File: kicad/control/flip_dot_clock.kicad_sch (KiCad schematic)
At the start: 34 parts, among them J1 Conn_01x02_Male, U1 NUCLEO-F303K8-HEADER, U10 Small_7_Seg_FlipDot_Module, U2 SLC03B-05, U3 NCV7719, U4 Small_7_Seg_FlipDot_Module, U5 NCV7719, U6 Small_7_Seg_FlipDot_Module, U7 NCV7719, U8 Small_7_Seg_FlipDot_Module, U9 NCV7719

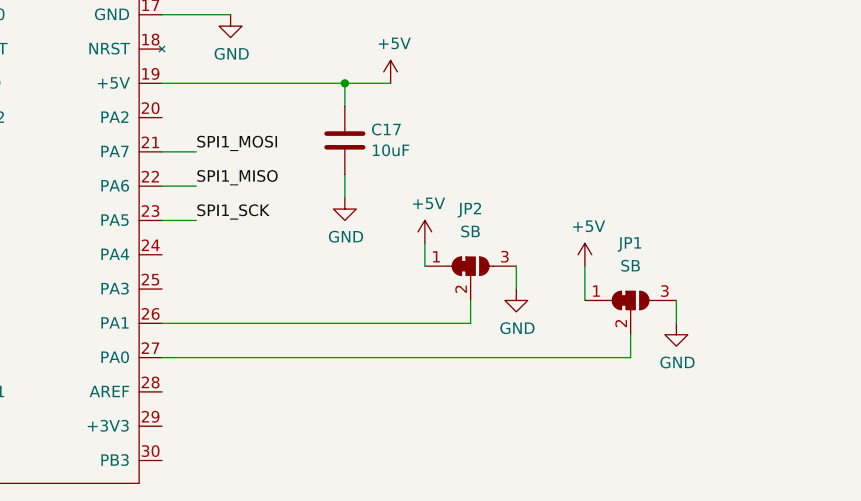
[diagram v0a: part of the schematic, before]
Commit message: updates
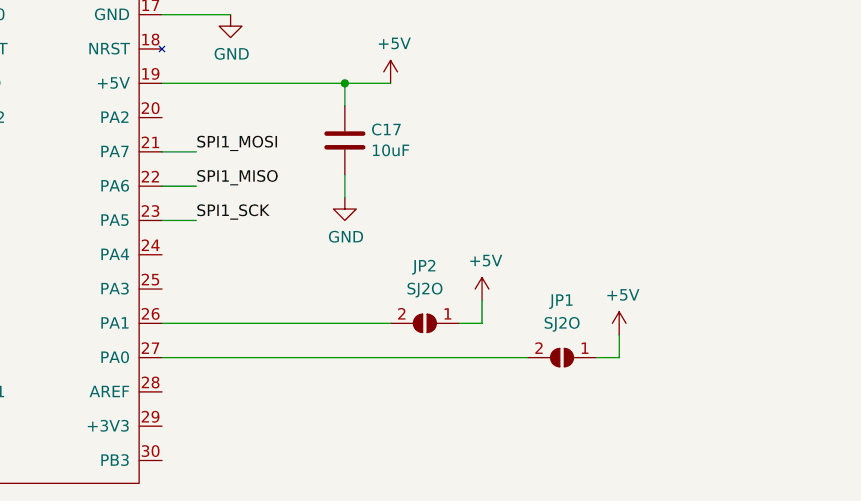
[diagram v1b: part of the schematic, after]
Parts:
- removed JP1, JP2: SB, Jumper:SolderJumper-3_P2.0mm_Open_TrianglePad1.0x1.5mm_NumberLabels, symbol Jumper:SolderJumper_3_Bridged12
- added JP1, JP2: SJ2O, Jumper:SolderJumper-2_P1.3mm_Open_TrianglePad1.0x1.5mm, symbol Jumper:SolderJumper_2_Open
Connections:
- net +5V: now also JP1.1 (A), JP2.1 (A)
- net at U1.26 (PA1): now also JP2.2 (B)
- net at U1.27 (PA0): now also JP1.2 (B)
